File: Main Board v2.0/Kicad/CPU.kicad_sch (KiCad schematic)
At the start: 4 parts, among them U1 Z80CPU, Y1 20MHz

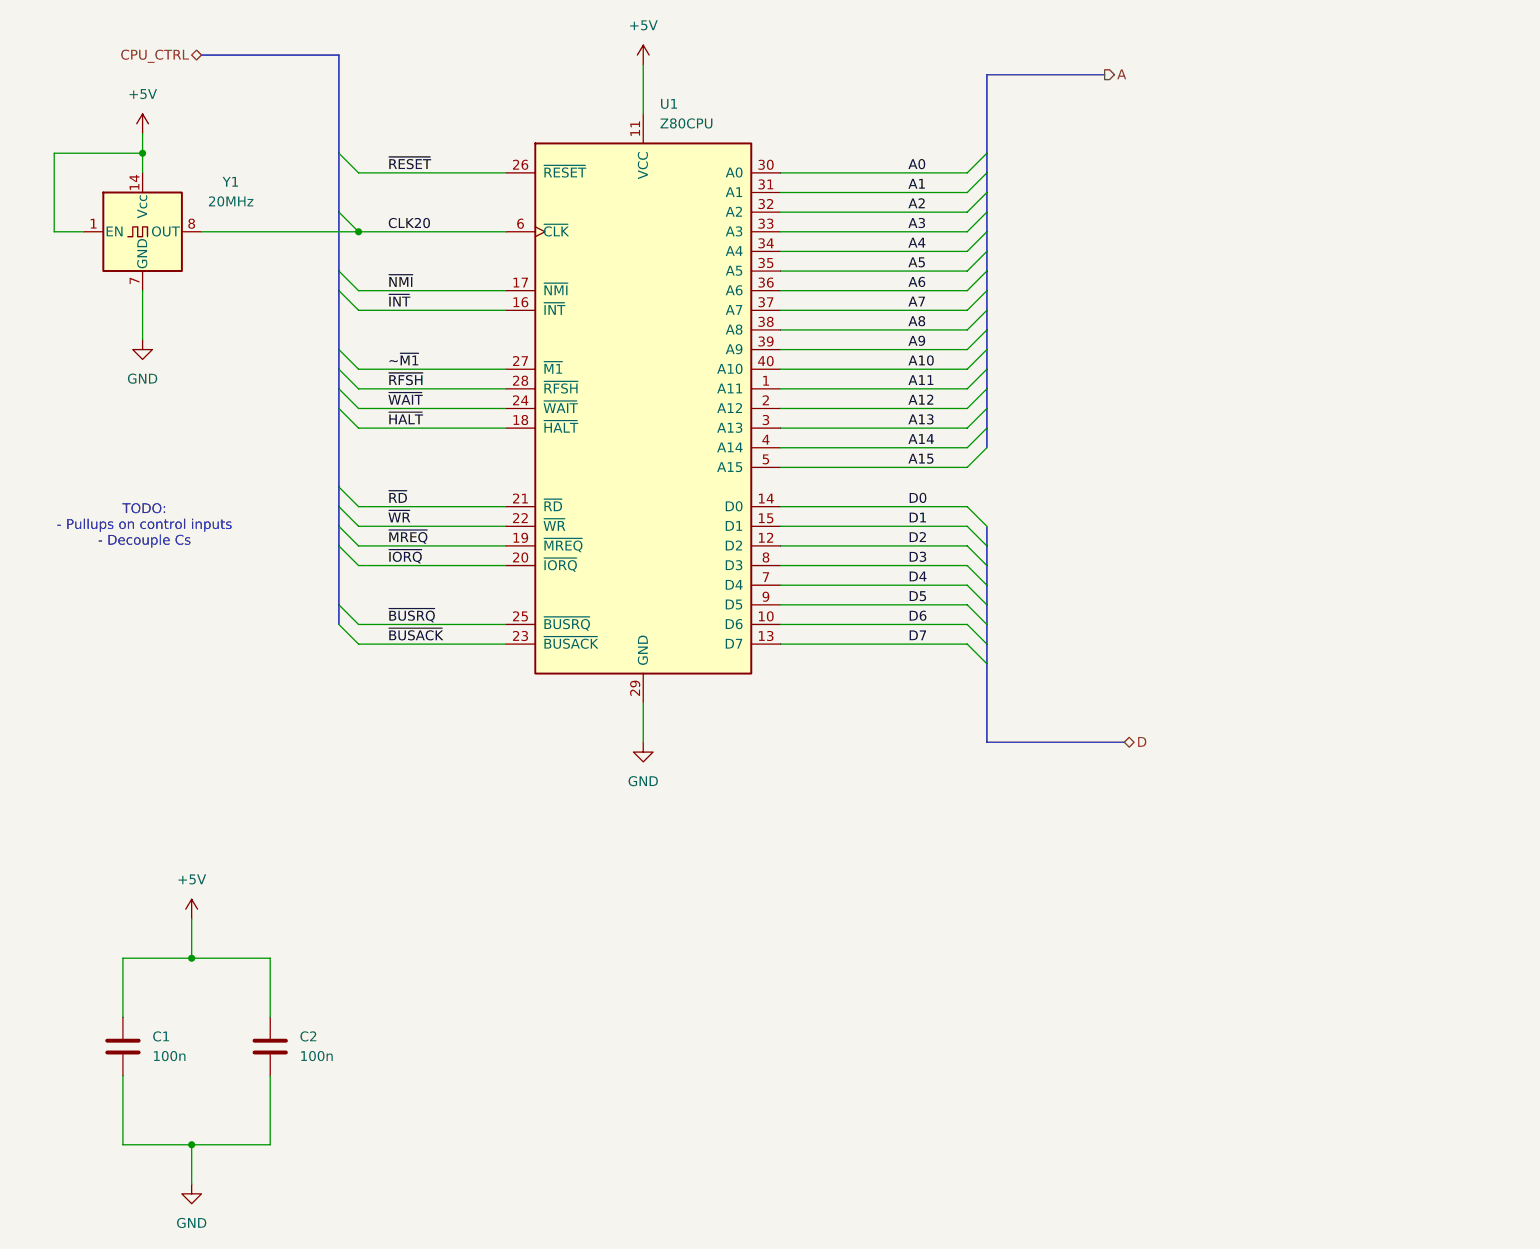
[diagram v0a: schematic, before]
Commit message: update
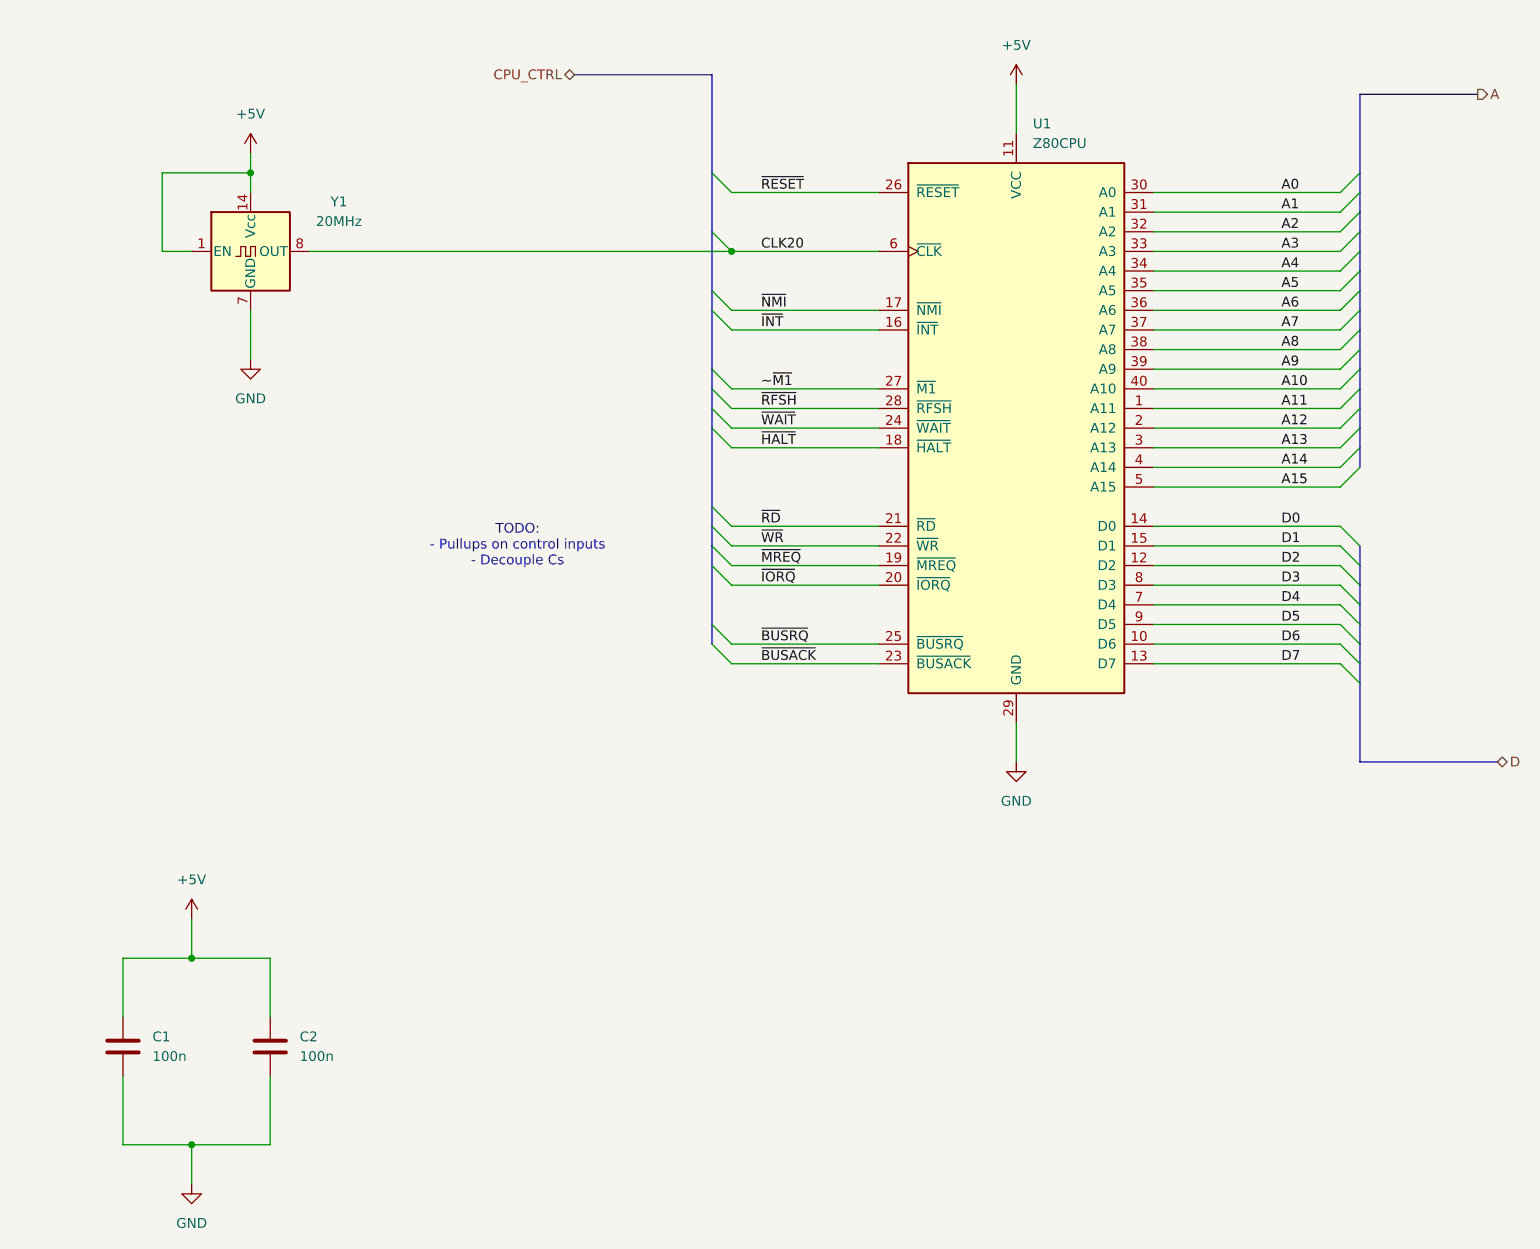
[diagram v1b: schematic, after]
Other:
- moved on the sheet: U1, Y1
